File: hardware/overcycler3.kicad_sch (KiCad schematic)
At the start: 127 parts, among them J1 USB_B, J2 AudioJack3_Switch, J3 DIN-5_180degree, J4 AudioJack3_Switch, J5 AudioJack3_Switch, P1 FT232, P2 PANEL, Q1 2SC945, SW1 RESET, SW2 POWER, U1 XT26G02ELGIGA, U2 TL074, U20 AD5328B, U3 LPC1778FBD144, U4 TLV2556, U5 74HC138, U6 TL074, U7 AD5328B, Y1 12MHz

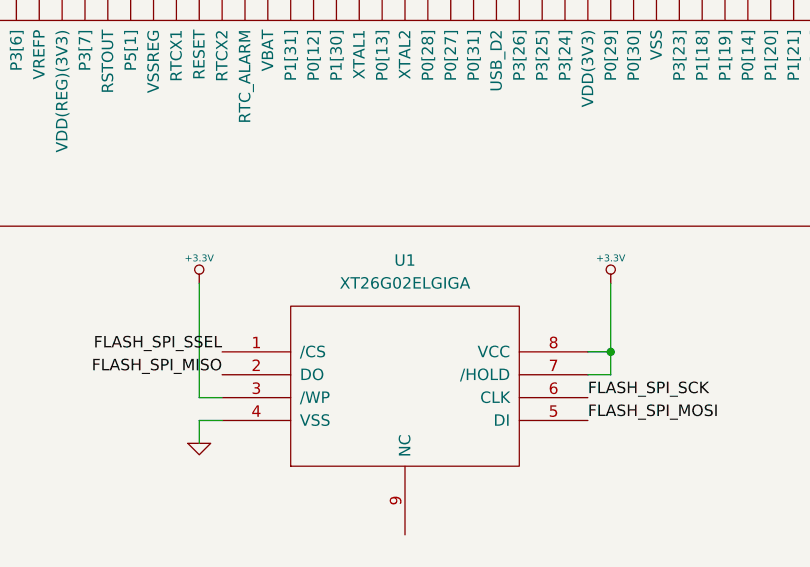
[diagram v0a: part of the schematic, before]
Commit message: hardware: proper production files for JLCPCB
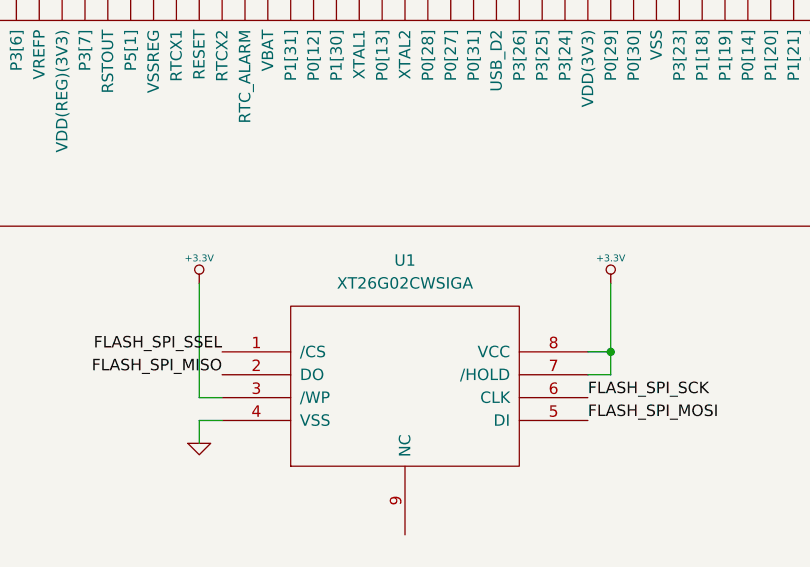
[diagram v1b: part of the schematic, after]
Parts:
- RV1: LCSC (none) -> C370979
- U1: value XT26G02ELGIGA -> XT26G02CWSIGA; footprint Package_LGA:LGA-8_8x6mm_P1.27mm -> Package_SON:WSON-8-1EP_8x6mm_P1.27mm_EP3.4x4.3mm
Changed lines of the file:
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@@
       (effects (font (size 1.27 1.27)))
     )
-    (property "Value" "XT26G02ELGIGA" (at 115.57 254 0)
-      (effects (font (size 1.27 1.27)))
-    )
-    (property "Footprint" "Package_LGA:LGA-8_8x6mm_P1.27mm" (at 115.57 265.43 0)
+    (property "Value" "XT26G02CWSIGA" (at 115.57 254 0)
+      (effects (font (size 1.27 1.27)))
+    )
+    (property "Footprint" "Package_SON:WSON-8-1EP_8x6mm_P1.27mm_EP3.4x4.3mm" (at 115.57 265.43 0)
       (effects (font (size 1.27 1.27)) hide)
     )
@@
       (effects (font (size 1.27 1.27)) hide)
     )
+    (property "LCSC" "C370979" (at 356.87 91.44 0)
+      (effects (font (size 1.27 1.27)) hide)
+    )

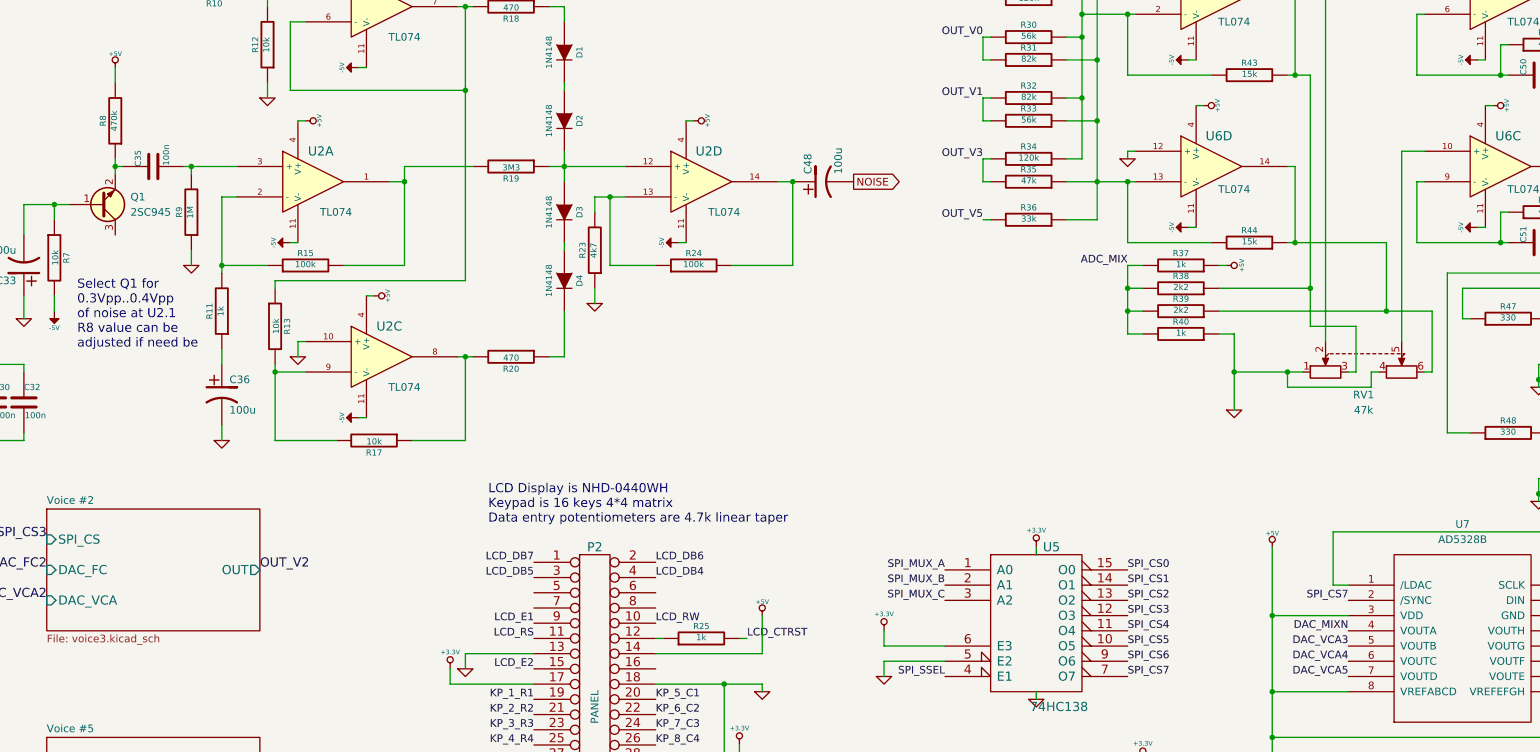
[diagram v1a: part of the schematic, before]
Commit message: hardware: oc3 hardware R2 (updates from porting the firmware)
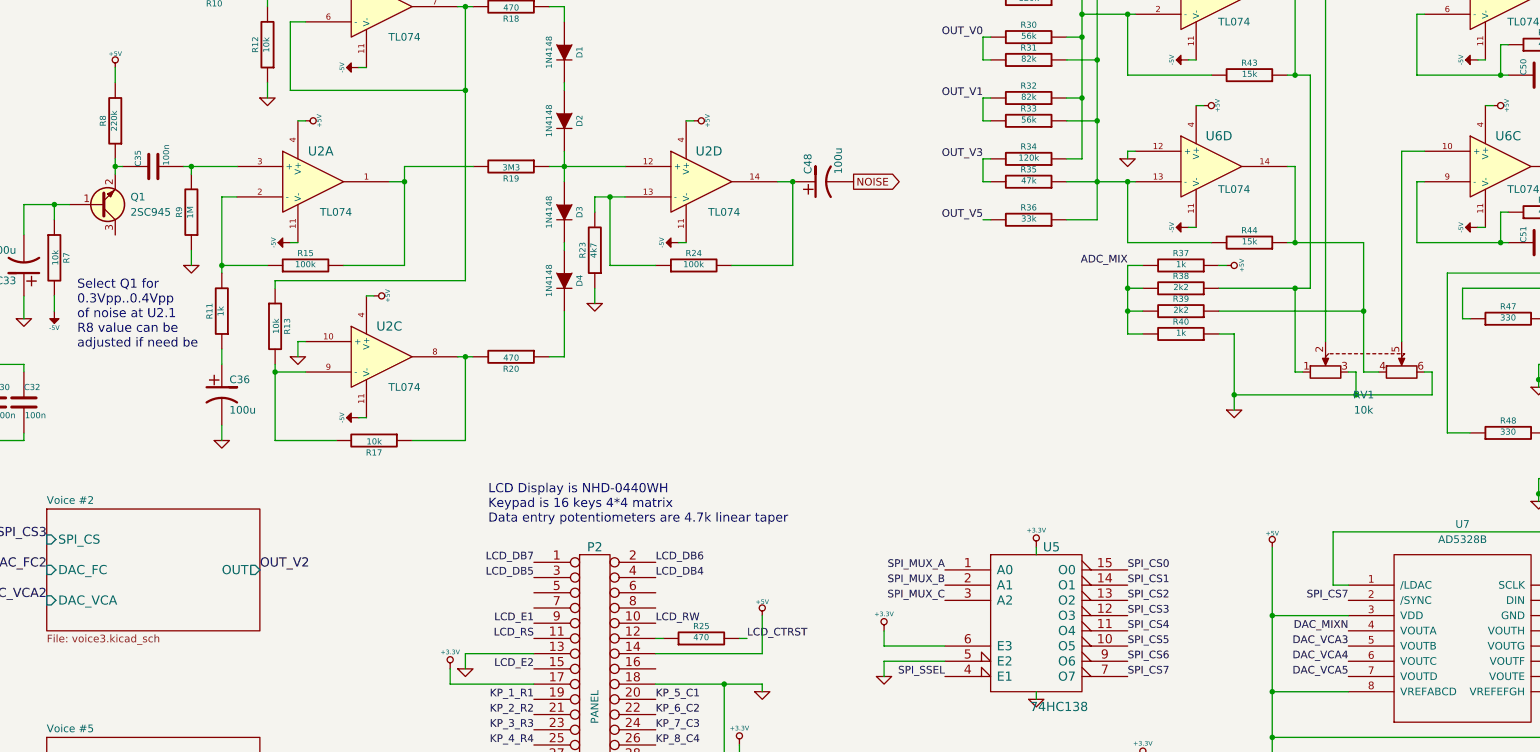
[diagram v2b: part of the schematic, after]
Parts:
- R25: value 1k -> 470; LCSC C17513 -> C17710
- R8: value 470k -> 220k; LCSC C17709 -> C17556
- RV1: value 47k -> 10k
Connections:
- net GND: now also RV1.3, RV1.6; no longer RV1.1, RV1.4
- net at R38.1, R43.1, U6.1: now also RV1.1; no longer RV1.3
- net at R39.1, R44.1, U6.14: now also RV1.4; no longer RV1.6
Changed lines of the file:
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@@
   (junction (at 29.21 73.66) (diameter 0) (color 0 0 0 0)
   )
-  (junction (at 335.28 87.63) (diameter 0) (color 0 0 0 0)
-  )
   (junction (at 55.88 62.23) (diameter 0) (color 0 0 0 0)
   )
@@
   (junction (at 64.77 73.66) (diameter 0) (color 0 0 0 0)
   )
+  (junction (at 356.87 77.47) (diameter 0) (color 0 0 0 0)
+  )
   (junction (at 196.85 55.88) (diameter 0) (color 0 0 0 0)
   )
@@
   (junction (at 118.11 99.06) (diameter 0) (color 0 0 0 0)
   )
+  (junction (at 345.44 73.66) (diameter 0) (color 0 0 0 0)
+  )
   (junction (at 19.05 195.58) (diameter 0) (color 0 0 0 0)
   )
@@
   (junction (at 320.04 189.23) (diameter 0) (color 0 0 0 0)
   )
-  (junction (at 344.17 87.63) (diameter 0) (color 0 0 0 0)
-  )
   (junction (at 184.15 271.78) (diameter 0) (color 0 0 0 0)
   )
-  (junction (at 360.68 77.47) (diameter 0) (color 0 0 0 0)
-  )
   (junction (at 345.44 38.1) (diameter 0) (color 0 0 0 0)
   )
@@
   (junction (at 386.08 88.9) (diameter 0) (color 0 0 0 0)
   )
-  (junction (at 347.98 73.66) (diameter 0) (color 0 0 0 0)
-  )
   (junction (at 312.42 45.72) (diameter 0) (color 0 0 0 0)
   )
@@
   (junction (at 34.29 35.56) (diameter 0) (color 0 0 0 0)
   )
+  (junction (at 355.6 91.44) (diameter 0) (color 0 0 0 0)
+  )
   (junction (at 34.29 86.36) (diameter 0) (color 0 0 0 0)
   )
@@
   (junction (at 44.45 86.36) (diameter 0) (color 0 0 0 0)
   )
+  (junction (at 335.28 91.44) (diameter 0) (color 0 0 0 0)
+  )
   (junction (at 200.66 181.61) (diameter 0) (color 0 0 0 0)
   )
@@
     (stroke (width 0) (type default))
   )
+  (wire (pts (xy 345.44 87.63) (xy 345.44 73.66))
+    (stroke (width 0) (type default))
+  )
   (wire (pts (xy 168.91 281.94) (xy 168.91 271.78))
     (stroke (width 0) (type default))
@@
     (stroke (width 0) (type default))
   )
-  (wire (pts (xy 344.17 87.63) (xy 346.71 87.63))
-    (stroke (width 0) (type default))
-  )
   (wire (pts (xy 198.12 99.06) (xy 207.01 99.06))
     (stroke (width 0) (type default))
@@
     (stroke (width 0) (type default))
   )
-  (wire (pts (xy 335.28 87.63) (xy 335.28 81.28))
-    (stroke (width 0) (type default))
-  )
   (wire (pts (xy 82.55 99.06) (xy 87.63 99.06))
     (stroke (width 0) (type default))
@@
     (stroke (width 0) (type default))
   )
-  (wire (pts (xy 344.17 90.17) (xy 358.14 90.17))
-    (stroke (width 0) (type default))
-  )
   (wire (pts (xy 189.23 95.25) (xy 190.5 95.25))
     (stroke (width 0) (type default))
@@
     (stroke (width 0) (type default))
   )
-  (wire (pts (xy 358.14 87.63) (xy 359.41 87.63))
-    (stroke (width 0) (type default))
-  )
   (wire (pts (xy 166.37 96.52) (xy 166.37 99.06))
     (stroke (width 0) (type default))
@@
     (stroke (width 0) (type default))
   )
+  (wire (pts (xy 359.41 87.63) (xy 356.87 87.63))
+    (stroke (width 0) (type default))
+  )
   (wire (pts (xy 328.93 43.18) (xy 330.2 43.18))
     (stroke (width 0) (type default))
@@
     (stroke (width 0) (type default))
   )
-  (wire (pts (xy 360.68 77.47) (xy 368.3 77.47))
-    (stroke (width 0) (type default))
-  )
   (wire (pts (xy 238.76 152.4) (xy 250.19 152.4))
     (stroke (width 0) (type default))
@@
     (stroke (width 0) (type default))
   )
-  (wire (pts (xy 344.17 87.63) (xy 344.17 90.17))
-    (stroke (width 0) (type default))
-  )
   (wire (pts (xy 175.26 87.63) (xy 180.34 87.63))
     (stroke (width 0) (type default))
@@
     (stroke (width 0) (type default))
   )
-  (wire (pts (xy 332.74 73.66) (xy 347.98 73.66))
+  (wire (pts (xy 332.74 73.66) (xy 345.44 73.66))
     (stroke (width 0) (type default))
   )
@@
     (stroke (width 0) (type default))
   )
+  (wire (pts (xy 335.28 91.44) (xy 335.28 93.98))
+    (stroke (width 0) (type default))
+  )
   (wire (pts (xy 92.71 269.24) (xy 95.25 269.24))
     (stroke (width 0) (type default))
@@
     (stroke (width 0) (type default))
   )
-  (wire (pts (xy 345.44 66.04) (xy 360.68 66.04))
+  (wire (pts (xy 345.44 66.04) (xy 356.87 66.04))
     (stroke (width 0) (type default))
   )
@@
     (stroke (width 0) (type default))
   )
+  (wire (pts (xy 354.33 87.63) (xy 355.6 87.63))
+    (stroke (width 0) (type default))
+  )
   (wire (pts (xy 205.74 162.56) (xy 218.44 162.56))
     (stroke (width 0) (type default))
@@
     (stroke (width 0) (type default))
   )
-  (wire (pts (xy 360.68 66.04) (xy 360.68 77.47))
-    (stroke (width 0) (type default))
-  )
   (wire (pts (xy 179.07 45.72) (xy 180.34 45.72))
     (stroke (width 0) (type default))
@@
     (stroke (width 0) (type default))
   )
+  (wire (pts (xy 368.3 87.63) (xy 367.03 87.63))
+    (stroke (width 0) (type default))
+  )
   (wire (pts (xy 220.98 53.34) (xy 223.52 53.34))
     (stroke (width 0) (type default))
@@
     (stroke (width 0) (type default))
   )
-  (wire (pts (xy 332.74 77.47) (xy 360.68 77.47))
-    (stroke (width 0) (type default))
-  )
   (wire (pts (xy 320.04 153.67) (xy 320.04 158.75))
     (stroke (width 0) (type default))
@@
     (stroke (width 0) (type default))
   )
-  (wire (pts (xy 355.6 80.01) (xy 347.98 80.01))
-    (stroke (width 0) (type default))
-  )
   (wire (pts (xy 19.05 193.04) (xy 19.05 195.58))
     (stroke (width 0) (type default))
@@
     (stroke (width 0) (type default))
   )
-  (wire (pts (xy 335.28 93.98) (xy 335.28 87.63))
+  (wire (pts (xy 335.28 81.28) (xy 335.28 91.44))
     (stroke (width 0) (type default))
   )
@@
     (stroke (width 0) (type default))
   )
+  (wire (pts (xy 356.87 66.04) (xy 356.87 77.47))
+    (stroke (width 0) (type default))
+  )
   (wire (pts (xy 223.52 85.09) (xy 223.52 77.47))
     (stroke (width 0) (type default))
@@
     (stroke (width 0) (type default))
   )
-  (wire (pts (xy 358.14 90.17) (xy 358.14 87.63))
-    (stroke (width 0) (type default))
-  )
   (wire (pts (xy 232.41 207.01) (xy 229.87 207.01))
     (stroke (width 0) (type default))
@@
     (stroke (width 0) (type default))
   )
+  (wire (pts (xy 332.74 77.47) (xy 356.87 77.47))
+    (stroke (width 0) (type default))
+  )
   (wire (pts (xy 184.15 281.94) (xy 189.23 281.94))
     (stroke (width 0) (type default))
@@
     (stroke (width 0) (type default))
   )
-  (wire (pts (xy 355.6 87.63) (xy 354.33 87.63))
-    (stroke (width 0) (type default))
-  )
   (wire (pts (xy 388.62 76.2) (xy 388.62 102.87))
     (stroke (width 0) (type default))
@@
     (stroke (width 0) (type default))
   )
+  (wire (pts (xy 355.6 91.44) (xy 335.28 91.44))
+    (stroke (width 0) (type default))
+  )
   (wire (pts (xy 19.05 177.8) (xy 19.05 180.34))
     (stroke (width 0) (type default))
@@
     (stroke (width 0) (type default))
   )
-  (wire (pts (xy 232.41 273.05) (xy 232.41 274.32))
+  (wire (pts (xy 355.6 87.63) (xy 355.6 91.44))
     (stroke (width 0) (type default))
   )
-  (wire (pts (xy 347.98 80.01) (xy 347.98 73.66))
+  (wire (pts (xy 232.41 273.05) (xy 232.41 274.32))
     (stroke (width 0) (type default))
   )
@@
     (stroke (width 0) (type default))
   )
-  (wire (pts (xy 368.3 87.63) (xy 368.3 77.47))
-    (stroke (width 0) (type default))
-  )
   (wire (pts (xy 309.88 27.94) (xy 317.5 27.94))
     (stroke (width 0) (type default))
@@
     (stroke (width 0) (type default))
   )
+  (wire (pts (xy 368.3 91.44) (xy 368.3 87.63))
+    (stroke (width 0) (type default))
+  )
   (wire (pts (xy 90.17 50.8) (xy 120.65 50.8))
     (stroke (width 0) (type default))
@@
     (stroke (width 0) (type default))
   )
+  (wire (pts (xy 356.87 77.47) (xy 356.87 87.63))
+    (stroke (width 0) (type default))
+  )
   (wire (pts (xy 20.32 260.35) (xy 17.78 260.35))
     (stroke (width 0) (type default))
   )
+  (wire (pts (xy 345.44 73.66) (xy 347.98 73.66))
+    (stroke (width 0) (type default))
+  )
   (wire (pts (xy 34.29 35.56) (xy 34.29 40.64))
     (stroke (width 0) (type default))
@@
     (stroke (width 0) (type default))
   )
+  (wire (pts (xy 355.6 91.44) (xy 368.3 91.44))
+    (stroke (width 0) (type default))
+  )
   (wire (pts (xy 39.37 86.36) (xy 44.45 86.36))
     (stroke (width 0) (type default))
@@
     (stroke (width 0) (type default))
   )
-  (wire (pts (xy 355.6 80.01) (xy 355.6 87.63))
-    (stroke (width 0) (type default))
-  )
   (wire (pts (xy 19.05 195.58) (xy 19.05 198.12))
     (stroke (width 0) (type default))
@@
     (stroke (width 0) (type default))
   )
-  (wire (pts (xy 335.28 87.63) (xy 344.17 87.63))
-    (stroke (width 0) (type default))
-  )
   (wire (pts (xy 317.5 77.47) (xy 317.5 73.66))
     (stroke (width 0) (type default))
@@
     (stroke (width 0) (type default))
   )
+  (wire (pts (xy 346.71 87.63) (xy 345.44 87.63))
+    (stroke (width 0) (type default))
+  )
   (wire (pts (xy 320.04 176.53) (xy 320.04 189.23))
     (stroke (width 0) (type default))
@@
     (stroke (width 0) (type default))
   )
-  (wire (pts (xy 368.3 87.63) (xy 367.03 87.63))
-    (stroke (width 0) (type default))
-  )
   (wire (pts (xy 252.73 132.08) (xy 254 132.08))
     (stroke (width 0) (type default))
@@
       (effects (font (size 1.016 1.016)))
     )
-    (property "Value" "470k" (at 148.4122 45.7454 90)
+    (property "Value" "220k" (at 148.4122 45.7454 90)
       (effects (font (size 1.016 1.016)))
     )
@@
       (effects (font (size 0.762 0.762)))
     )
-    (property "LCSC" "C17709" (at 146.558 45.72 0)
+    (property "LCSC" "C17556" (at 146.558 45.72 0)
       (effects (font (size 1.27 1.27)) hide)
     )
@@
       (effects (font (size 1.27 1.27)))
     )
-    (property "Value" "47k" (at 356.87 93.98 0)
+    (property "Value" "10k" (at 356.87 93.98 0)
       (effects (font (size 1.27 1.27)))
     )
@@
       (effects (font (size 1.016 1.016)))
     )
-    (property "Value" "1k" (at 246.3546 131.9022 90)
+    (property "Value" "470" (at 246.3546 131.9022 90)
       (effects (font (size 1.016 1.016)))
     )
@@
       (effects (font (size 0.762 0.762)))
     )
-    (property "LCSC" "C17513" (at 246.38 130.048 0)
+    (property "LCSC" "C17710" (at 246.38 130.048 0)
       (effects (font (size 1.27 1.27)) hide)
     )
